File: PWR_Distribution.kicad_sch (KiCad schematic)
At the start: 42 parts, among them J1 CarPowerConnector, U22 AP64501SP-13, U7 LM76202QPWPRQ1

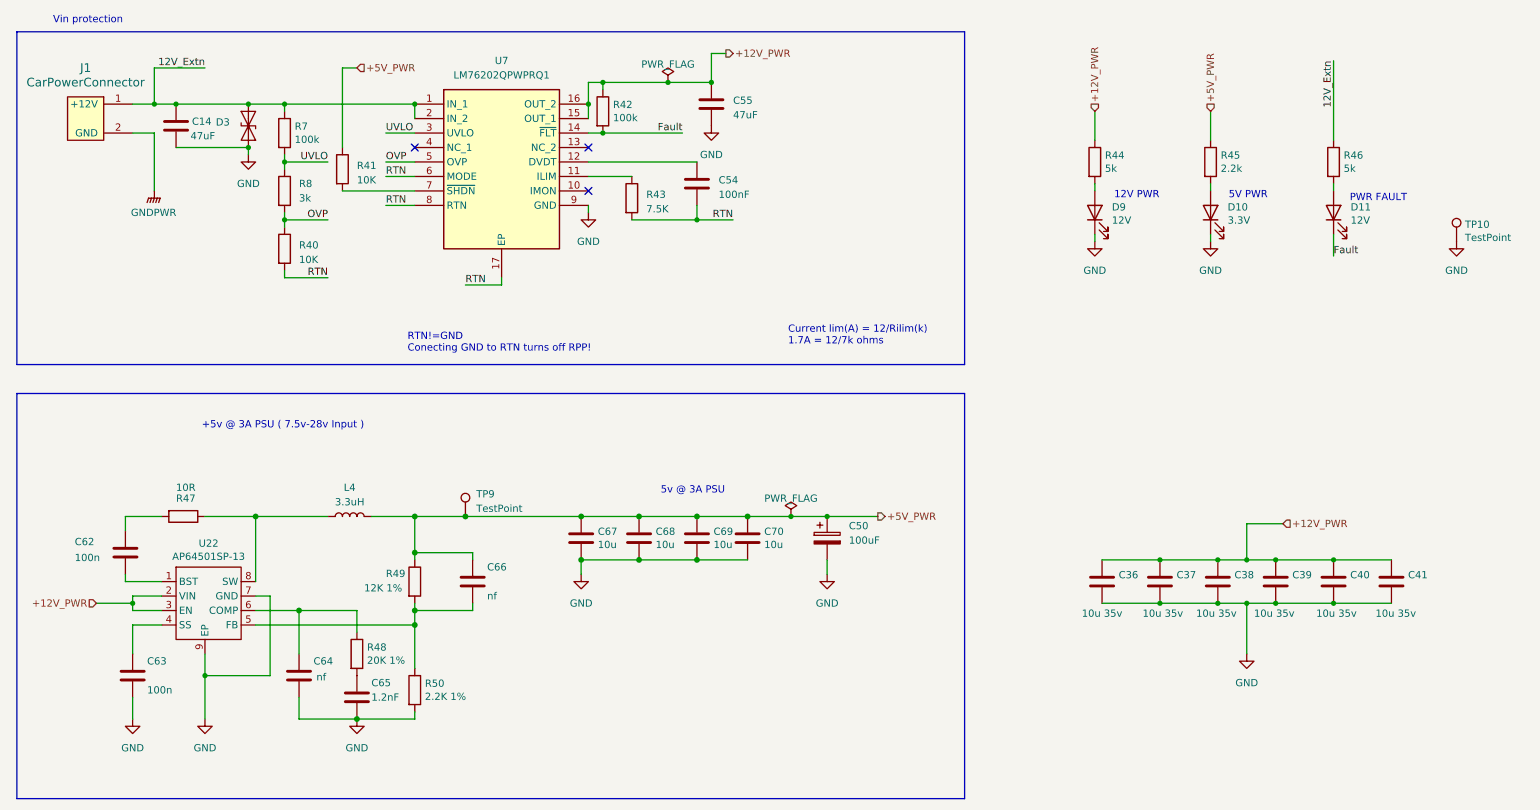
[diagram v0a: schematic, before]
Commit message: think im done with schematic
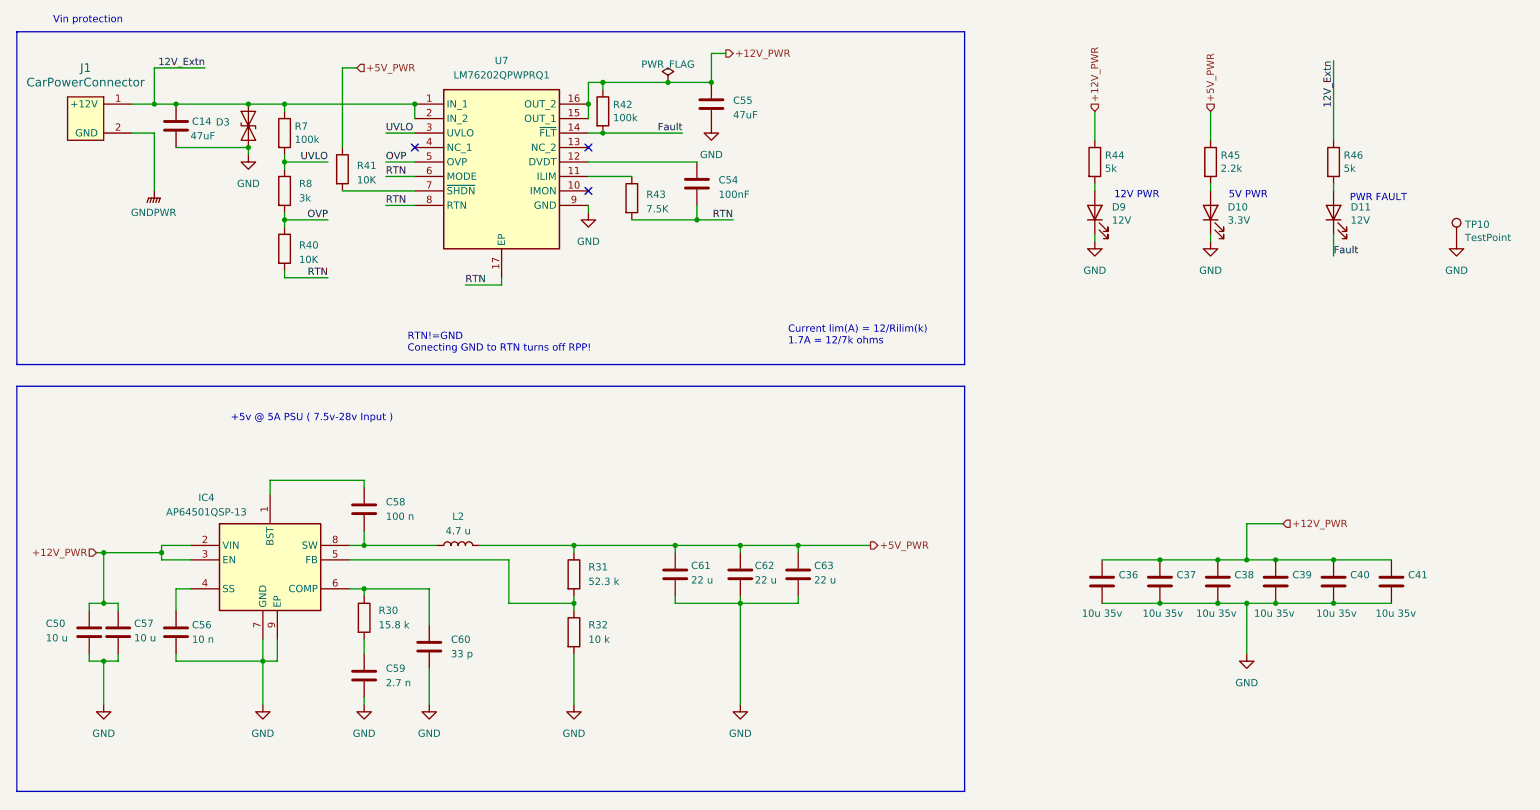
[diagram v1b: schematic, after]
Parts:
- removed C50: 100uF, symbol Device:C_Polarized
- removed C64, C66: nf, Capacitor_SMD:C_0402_1005Metric, symbol Device:C
- removed C65: 1.2nF, Capacitor_SMD:C_0402_1005Metric, symbol Device:C
- removed C67, C68, C69, C70: 10u, Capacitor_SMD:C_0805_2012Metric, symbol Device:C
- removed L4: 3.3uH, symbol Device:L
- removed R47: 10R, Resistor_SMD:R_0402_1005Metric, symbol Device:R
- removed R48: 20K 1%, Resistor_SMD:R_0402_1005Metric, symbol Device:R
- removed R49: 12K 1%, Resistor_SMD:R_0402_1005Metric, symbol Device:R
- removed R50: 2.2K 1%, Resistor_SMD:R_0402_1005Metric, symbol Device:R
- removed TP9: TestPoint, TestPoint:TestPoint_Pad_2.0x2.0mm, symbol Connector:TestPoint
- removed U22: AP64501SP-13, Package_SO:SOIC-8-1EP_3.9x4.9mm_P1.27mm_EP2.95x4.9mm_Mask2.71x3.4mm_ThermalVias, symbol CM4IO:AP64351
- added C50, C57: 10 u, symbol Device:C
- added C56: 10 n, symbol Device:C
- added C58: 100 n, symbol Device:C
- added C59: 2.7 n, symbol Device:C
- added C60: 33 p, symbol Device:C
- added C61: 22 u, symbol Device:C
- added IC4: AP64501QSP-13, SOIC127P600X163-9N, symbol AP64501QSP-13:AP64501QSP-13
- added L2: 4.7 u, symbol Device:L
- added R30: 15.8 k, symbol Device:R
- added R31: 52.3 k, symbol Device:R
- added R32: 10 k, symbol Device:R
- C62, C63: value 100n -> 22 u; footprint Capacitor_SMD:C_0402_1005Metric -> (none); Field4 Farnell -> (none); Field5 2611911 -> (none); Field6 RM EMK105 B7104KV-F -> (none); Field7 TAIYO YUDEN EUROPE GMBH -> (none); Field8 110091611 -> (none); Part Description 0.1uF 10% 16V Ceramic Capacitor X7R 0402 (1005 Metric) -> (none)
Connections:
- net +12V_PWR: now also C50.1, C57.1, IC4.2 (VIN), IC4.3 (EN)
- net +5V_PWR: now also C62.1, C63.1, C61.1, L2.2, R31.1
- net GND: now also C62.2, C50.2, C56.2, C57.2, C59.2, C60.2, C61.2, IC4.7 (GND), IC4.9 (EP), R32.2
- new net: C60.1, IC4.6 (COMP), R30.1
- new net: C59.1, R30.2
- new net: C56.1, IC4.4 (SS)
- new net: C58.1, IC4.1 (BST)
- new net: C58.2, IC4.8 (SW), L2.1
- new net: IC4.5 (FB), R31.2, R32.1
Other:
- note added: "+5v @ 5A PSU ( 7.5v-28v Input )"
- note removed: "+5v @ 3A PSU ( 7.5v-28v Input )"
- note removed: "5v @ 3A PSU"
